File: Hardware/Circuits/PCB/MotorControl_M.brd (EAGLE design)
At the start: 72 x 150 mm, 72 parts, among them U1 LTC4359CMS8PBF, U2 SX1509, U3 MAX8881EUT50T

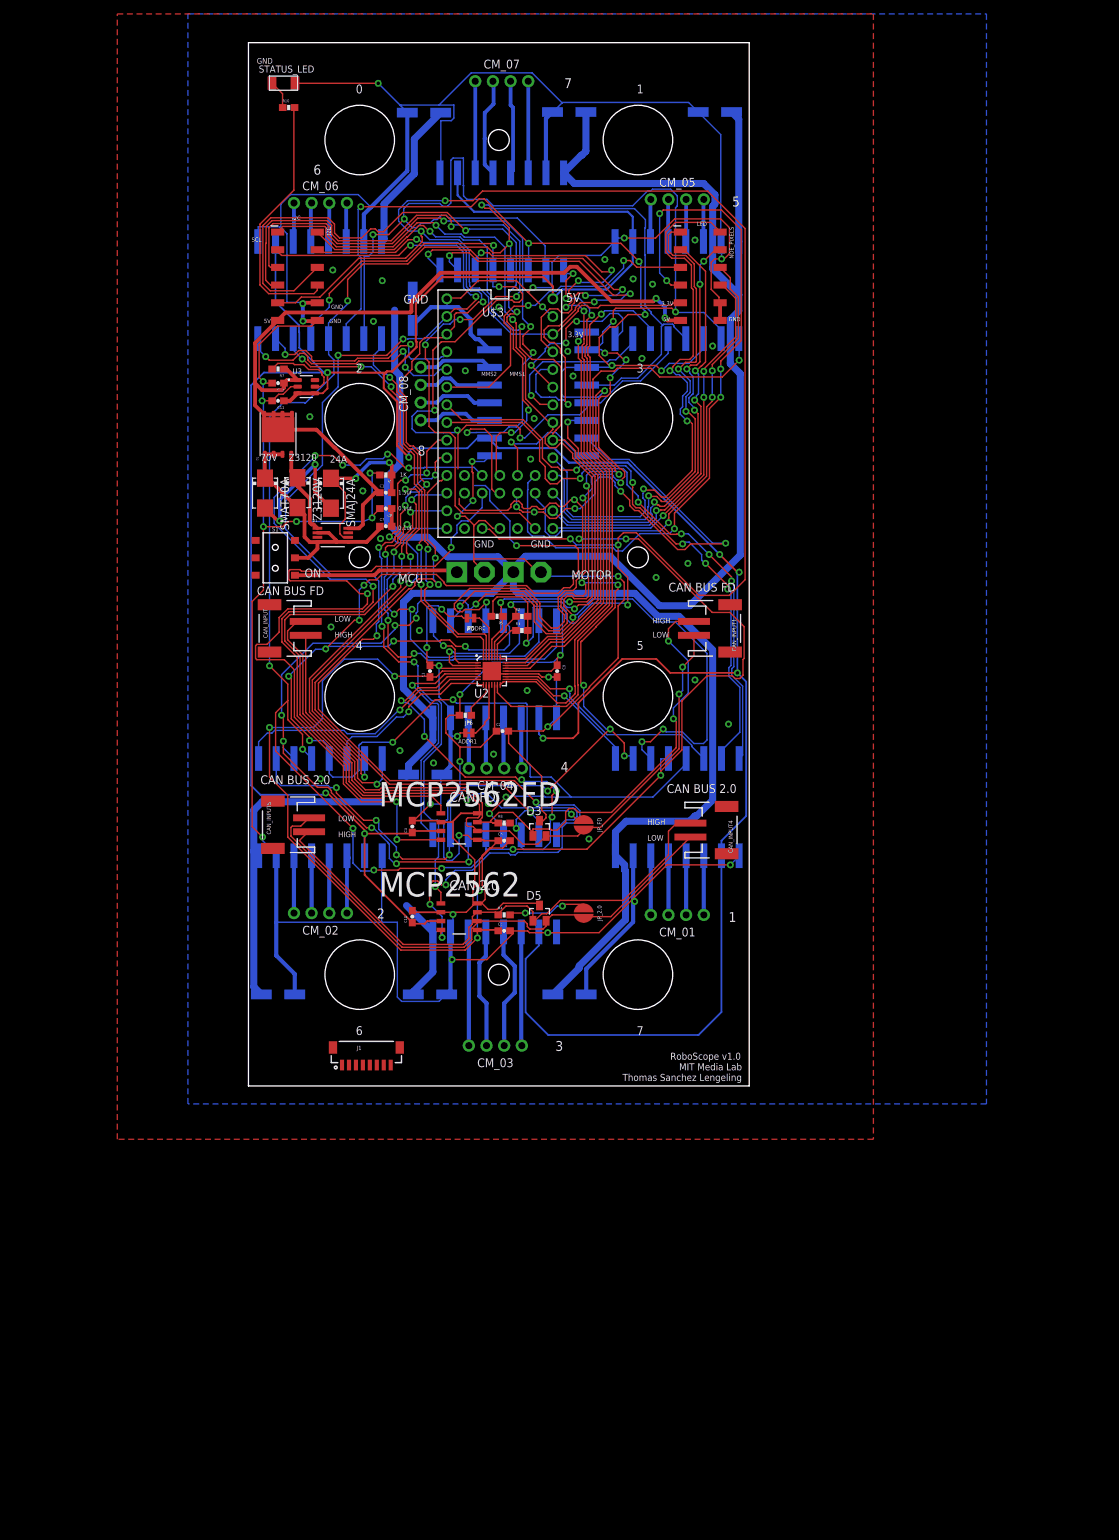
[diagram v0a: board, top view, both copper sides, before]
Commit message: update circuits
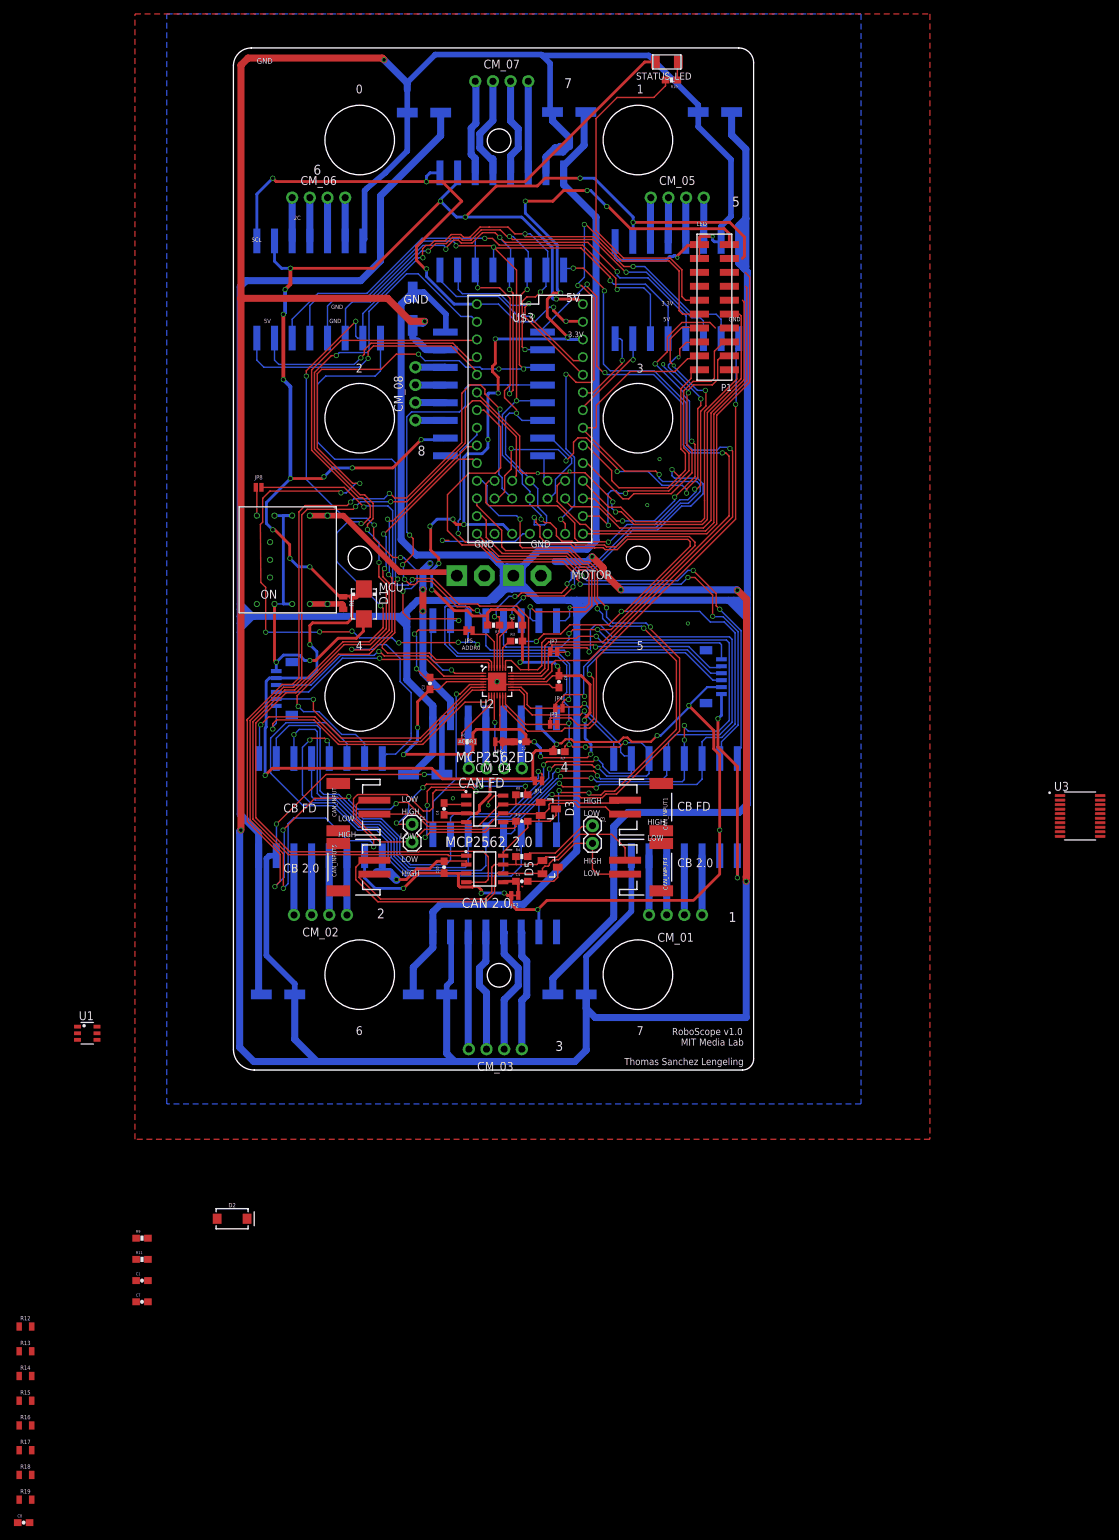
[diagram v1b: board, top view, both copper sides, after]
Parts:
- removed C11, C12: 4.7uf, SparkFun-Capacitors:0603-CAP
- removed I2C, NOE_PIXELS: (no value), SparkFun-Connectors:2X6_SMD
- removed JP_2.0, JP_FD: JUMPER-SMT_2_NO_NO-SILK_ROUND, SparkFun-Jumpers:SMT-JUMPER_2_NO_NO-SILK_ROUND
- removed MCP2562: MCP2562, MCP2562:MCP2562
- removed S1: (no value), SparkFun-Switches:SWITCH_DPDT_SMD_AYZ0202
- removed SMAJ24A, SMAT70A, Z3120V: S2M, s2x_10:DO214AA
- added D2: 3A/40V/500mV, SparkFun-DiscreteSemi:SMA-DIODE
- added J2, J3: (no value), SparkFun-Connectors:1X02
- added J4: (no value), SparkFun-Connectors:1X06-1MM
- added JP1, JP2: JUMPER-SMT_2_NC_TRACE_NO-SILK, SparkFun-Jumpers:SMT-JUMPER_2_NC_TRACE_NO-SILK
- added JP3, JP4, JP7: SMT_2, SparkFun-Jumpers:SMT-JUMPER_2_NC_TRACE_NO-SILK
- added JP8: SMT_2, SparkFun-Jumpers:SMT-JUMPER_2_NO_NO-SILK
- added MCP2562_2.0: MCP2562-E/SN, MCP2562-E_SN:SOIC127P600X175-8N
- added P1: M-2X10-87759, con-headers-jp:87759-20
- added R11, R9: 10K, SparkFun-Resistors:0603-RES
- added R12, R13, R14, R15, R16, R17, R18, R19: 100, SparkFun-Resistors:0805
- added U$1: MOSFET_SLIDER, Mosfet_slider:MOSFET_SLIDER
- C1: value 1.5uf -> 47uf/10V
- D1: value BSC010NE2LSI -> S2A; device BSC010NE2LSI:SOFL127P515X615X110-9N -> s2x_10:DO214AA
- J1: device SparkFun-Connectors:BM08B-SRSS-TB -> SparkFun-Connectors:1X06-1MM
- MCP2562FD: value MCP2562 -> MCP2562-E/SN; device MCP2562:MCP2562 -> MCP2562-E_SN:SOIC127P600X175-8N
- R1: value 1K -> 0.3; device SparkFun-Resistors:0603-RES -> SparkFun-Resistors:0805
- R7: value 100K -> 120Ohms
- U1: value LTC4359CMS8PBF -> MIC2005; device LTC4359CMS8PBF:MSOP-8_MS -> Microchip:SOT23-6
- U3: value MAX8881EUT50T -> TEXAS_INSTRUMENTS_SN74HCT245DW; device MAX8881EUT50T:SOT95P280X145-6N -> Texas Instruments - SN74HCT245DW:74HCT245
- moved C8 154.8 mm to (-30.2, -59.7), turned to 0 degrees
- moved U3 127.2 mm to (121.7, 41.9)
- moved C1 118.6 mm to (-13.2, -24.9)
- moved C7 116.9 mm to (-13.2, -27.9)
- moved U1 79.9 mm to (-21.1, 10.7)
- moved R7 68.2 mm to (46.7, 51.2)
- moved J1 55.3 mm to (7.37, 60.2), flipped to the bottom, turned to 270 degrees
- moved STATUS_LED 55.2 mm to (62.3, 150.3), turned to 180 degrees
- moved R10 55.2 mm to (62.9, 147.7), turned to 180 degrees
- moved CAN_INPUT1 27.5 mm to (59.9, 43.2)
- moved CAN_INPUT 27.5 mm to (16.5, 43.2)
- moved D1 27.3 mm to (18.7, 72.4), turned to 270 degrees
- moved R1 19.4 mm to (15.7, 72.5), turned to 270 degrees
- moved CAN_INPUT5 11.2 mm to (16.5, 34.5)
- moved CAN_INPUT4 10.8 mm to (59.9, 34.5)
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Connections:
- removed net N$12: SMAJ24A.A, SMAT70A.A
- removed net TRQ1: MOTOR_01.1, MOTOR_02.1, MOTOR_03.1, MOTOR_04.1, MOTOR_05.1, MOTOR_06.1, MOTOR_07.1, MOTOR_08.1, U$3.28
- removed net TRQ2: MOTOR_01.2, MOTOR_02.2, MOTOR_03.2, MOTOR_04.2, MOTOR_05.2, MOTOR_06.2, MOTOR_07.2, MOTOR_08.2, U$3.29
- removed net VCC_5V: C1.1, C12.1, D1.5, D1.6, D1.7, D1.8, D1.9, I2C.11, J1.2, NOE_PIXELS.11, R7.1, U1.8, U3.1
- new net CLK_RX/STANBY: MOTOR_01.STBY, MOTOR_02.STBY, MOTOR_03.STBY, MOTOR_04.STBY, MOTOR_05.STBY, MOTOR_06.STBY, MOTOR_07.STBY, MOTOR_08.STBY, U$3.29
- new net N$10: R11.2, U1.4
- new net N$11: R12.2, U3.18
- new net N$13: R9.2, U1.3
- new net N$21: R13.2, U3.17
- new net N$22: R14.2, U3.16
- new net N$23: R15.2, U3.15
- new net N$25: R17.2, U3.13
- new net N$26: R18.2, U3.12
- new net N$27: R19.2, U3.11
- new net N$5: C6.1, JP1.1, MCP2562FD.5
- new net N$7: U$1.GND_5
- new net N$8: P1.16
- new net NEOPIXEL_01_5V: P1.1, R12.1
- new net NEOPIXEL_02_5V: P1.3, R13.1
- new net NEOPIXEL_03_5V: P1.5, R14.1
- new net NEOPIXEL_04_5V: P1.7, R15.1
- new net NEOPIXEL_05_5V: P1.9, R16.1
- new net NEOPIXEL_06_5V: P1.11, R17.1
- new net NEOPIXEL_07_5V: P1.13, R18.1
- new net NEOPIXEL_08_5V: P1.15, R19.1
- new net TRQ1_SPREAD: JP7.2, MOTOR_01.1, MOTOR_02.1, MOTOR_03.1, MOTOR_04.1, MOTOR_05.1, MOTOR_06.1, MOTOR_07.1, MOTOR_08.1
- new net TRQ2/UART: MOTOR_01.2, MOTOR_02.2, MOTOR_03.2, MOTOR_04.2, MOTOR_05.2, MOTOR_06.2, MOTOR_07.2, MOTOR_08.2, U$3.28
- new net VCC_LEDS: C1.1, C7.1, D1.C, D2.A, D2.C, P1.17, R1.1, U1.1
- net 3.3V: now also P1.19; no longer C5.1, C6.1, I2C.9, MCP2562.VIO, MCP2562FD.VIO, NOE_PIXELS.9
- net CAN_H: now also MCP2562FD.7; no longer MCP2562FD.CANH
- net CAN_H2: now also MCP2562_2.0.7; no longer MCP2562.CANH
- net CAN_L: now also J2.2, MCP2562FD.6; no longer JP_FD.2, MCP2562FD.CANL
- net CAN_L2: now also J3.2, MCP2562_2.0.6; no longer JP_2.0.2, MCP2562.CANL
- net CAN_RX2: now also MCP2562_2.0.4; no longer I2C.3, MCP2562.RXD
- net CAN_RX3: now also MCP2562FD.4; no longer MCP2562FD.RXD
- net CAN_TX2: now also MCP2562_2.0.1; no longer I2C.4, MCP2562.TXD
- net CAN_TX3: now also MCP2562FD.1; no longer MCP2562FD.TXD
- net GND_MCU: now also C1.2, C7.2, D1.A, J4.1, MCP2562FD.2, MCP2562FD.8, MCP2562_2.0.2, MCP2562_2.0.8, P1.18, P1.20, U$1.GND_1, U$1.GND_2, U$1.GND_3, U$1.GND_4, U1.2, U3.10, U3.19; no longer C11.2, C12.2, I2C.10, I2C.12, MCP2562.STBY, MCP2562.VSS, MCP2562FD.STBY, MCP2562FD.VSS, NOE_PIXELS.10, NOE_PIXELS.12, R1.2, U3.2
- net INT_01: now also P1.6; no longer I2C.5
- net INT_02: now also P1.8; no longer I2C.6
- net MMS1: now also JP4.2
- net MMS2: now also JP3.2, R7.1
- net N$1: now also J2.1; no longer JP_FD.1
- net N$2: now also JP8.1, U$1.ON; no longer D1.4, U1.1, Z3120V.C
- net N$3: now also J3.1; no longer JP_2.0.1
- net N$4: now also R16.2, U3.14; no longer C1.2, R1.1, SMAJ24A.C, U1.6
- net N$6: now also C5.1, JP2.1, MCP2562_2.0.5; no longer R7.2, U3.5
- net N$9: now also P1.14; no longer C7.2, C8.1
- net NEOPIXEL_01: now also U3.2; no longer NOE_PIXELS.1
- net NEOPIXEL_02: now also U3.3; no longer NOE_PIXELS.2
- net NEOPIXEL_03: now also U3.4; no longer NOE_PIXELS.3
- net NEOPIXEL_04: now also U3.5; no longer NOE_PIXELS.4
- net NEOPIXEL_05: now also U3.6; no longer NOE_PIXELS.5
- net NEOPIXEL_06: now also U3.7; no longer NOE_PIXELS.6
- net NEOPIXEL_07: now also U3.8; no longer NOE_PIXELS.7
- net NEOPIXEL_08: now also U3.9; no longer NOE_PIXELS.8
- net RESET: now also P1.10; no longer I2C.7
- net STATUS_PIN: now also P1.12; no longer I2C.8
- net SX00_1: now also J1.3; no longer J1.8, MOTOR_06.STBY
- net SX00_11: now also J4.4, JP4.1; no longer J1.3, MOTOR_01.STBY
- net SX00_13: now also J4.5, JP7.1; no longer MOTOR_07.STBY
- net SX00_15: now also J4.6, JP8.2; no longer MOTOR_08.STBY
- net SX00_3: now also J1.4; no longer J1.6, MOTOR_04.STBY
- net SX00_5: no longer MOTOR_03.STBY
- net SX00_7: now also J1.6; no longer J1.4, MOTOR_02.STBY
- net SX00_9: now also J4.3, JP3.1; no longer J1.7, MOTOR_05.STBY
- net SX00_SCL: now also P1.4; no longer I2C.1
- net SX00_SDA: now also P1.2; no longer I2C.2
- net VCC_5VREG: now also C8.1, J1.2, J4.2, JP1.2, JP2.2, MCP2562FD.3, MCP2562_2.0.3, R7.2, U1.6, U3.1, U3.20; no longer C11.1, MCP2562.VDD, MCP2562FD.VDD, U3.3, U3.4
- net VCC_MCU: now also U$1.VIN_1, U$1.VIN_2; no longer S1.3
- net VCC_SWITCH: now also R1.2, R11.1, R9.1, U$1.VOUT_1, U$1.VOUT_2; no longer C7.1, D1.1, D1.2, D1.3, S1.2, SMAT70A.C, U1.2, U1.4, U1.5, Z3120V.A
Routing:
- net TRQ1: track 393.1 -> 0.00 mm, vias 14 -> 0
- net TRQ2: track 346.3 -> 0.00 mm, vias 18 -> 0
- net CLK_RX/STANBY: track 0.00 -> 329.3 mm, vias 0 -> 9
- net TRQ2/UART: track 0.00 -> 317.0 mm, vias 0 -> 13
- net TRQ1_SPREAD: track 0.00 -> 305.2 mm, vias 0 -> 13
- net VCC_M: track 441.6 -> 717.2 mm
- net 3.3V: track 469.7 -> 245.9 mm, vias 14 -> 21
- net GND_MCU: track 760.1 -> 964.8 mm, vias 62 -> 33
- net VCC_5V: track 125.2 -> 0.00 mm, vias 2 -> 0
- net CAN_H: track 110.4 -> 40.1 mm, vias 2 -> 0
- net SX00_13: track 96.2 -> 35.4 mm, vias 5 -> 1
- net CAN_L: track 108.2 -> 48.4 mm, vias 2 -> 0
- net MSTEP_08: track 67.9 -> 12.8 mm, vias 5 -> 0
- net SX00_15: track 47.9 -> 100.2 mm, vias 1 -> 3
- net CAN_RX2: track 209.6 -> 158.0 mm, vias 9 -> 3
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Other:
- board size 72 x 150 mm -> 74.8 x 147 mm
- board text added: "CB 2.0"
- board text added: "CB FD"
- board text removed: "0.1uf"
- board text removed: "1.5uf"
- board text removed: "1K"
- board text removed: "24A"
- board text removed: "70V"
- board text removed: "CAN BUS 2.0"
- board text removed: "CAN BUS FD"
- board text removed: "MMS1"
- board text removed: "MMS2"
- board text removed: "Z3120"
